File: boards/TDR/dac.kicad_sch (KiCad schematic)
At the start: 9 parts, among them U15 MCP4822, U4 TLV3541

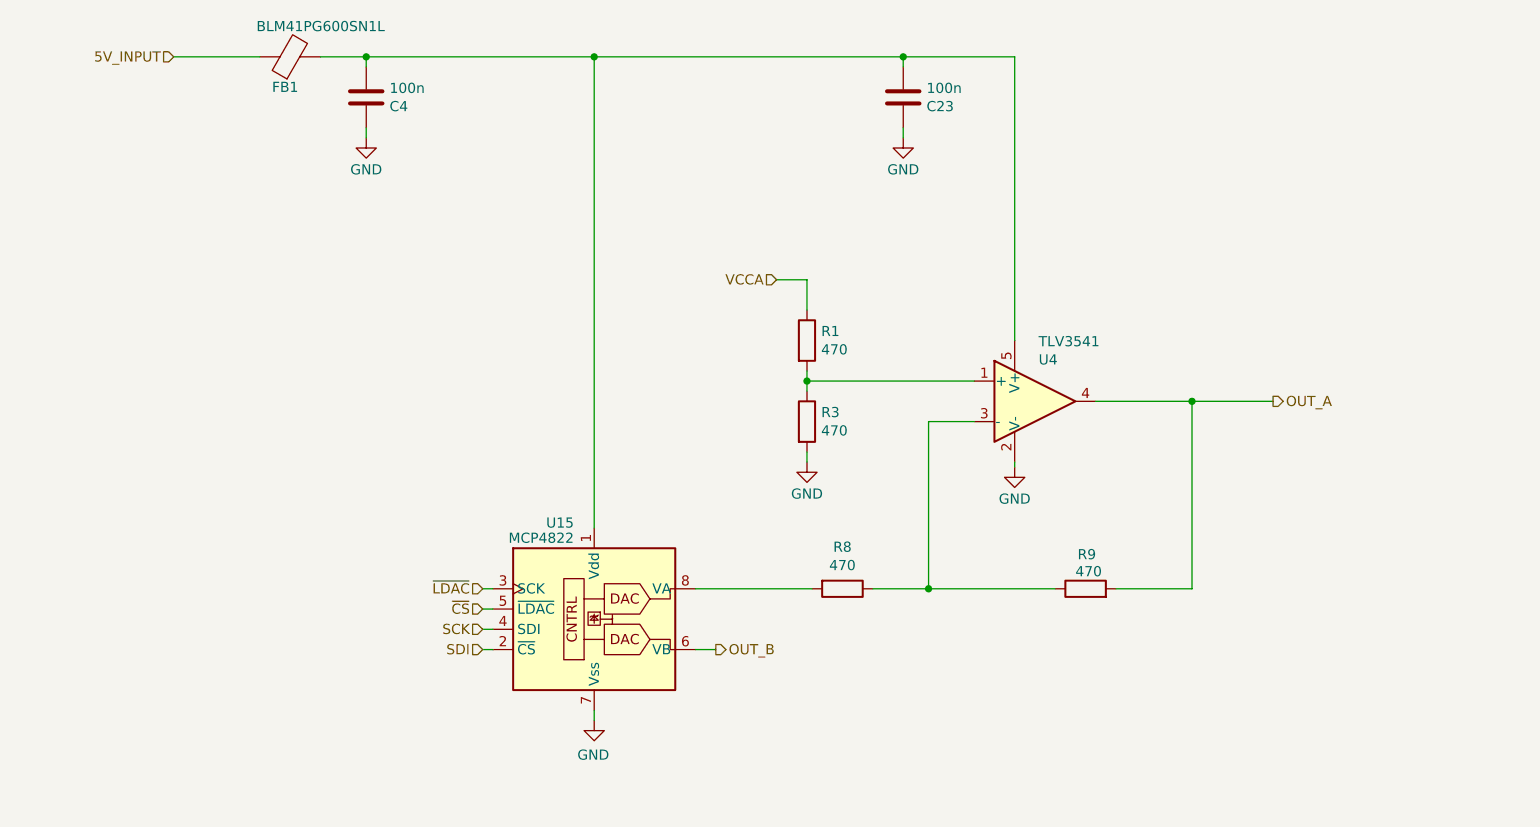
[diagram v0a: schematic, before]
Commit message: hopefully PCB is done
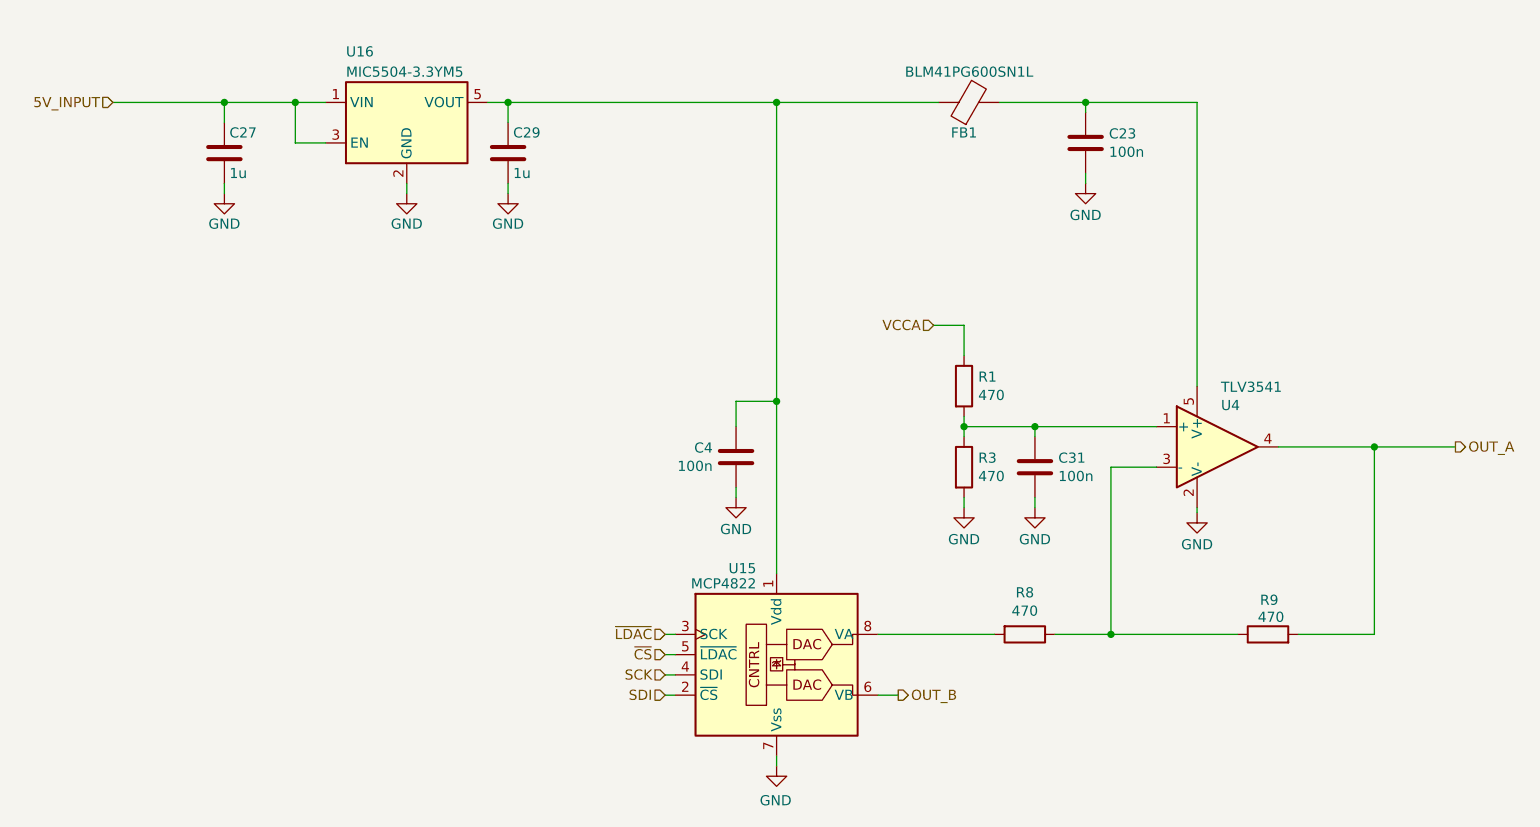
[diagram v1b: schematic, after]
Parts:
- added C27, C29: 1u, Capacitor_SMD:C_0805_2012Metric, symbol Device:C
- added C31: 100n, Capacitor_SMD:C_0402_1005Metric, symbol Device:C
- added U16: MIC5504-3.3YM5, Package_TO_SOT_SMD:SOT-23-5, symbol Regulator_Linear:MIC5504-3.3YM5
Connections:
- net 5V_INPUT: now also C27.1, U16.1 (VIN), U16.3 (EN); no longer FB1.1
- net GND: now also C27.2, C29.2, C31.1, U16.2 (GND)
- net at R1.2, R3.1, U4.1 (+): now also C31.2
- net at C23.1, FB1.2, U4.5 (V+): no longer C4.1, U15.1 (Vdd)
- new net: C29.1, C4.1, FB1.1, U15.1 (Vdd), U16.5 (VOUT)
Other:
- moved on the sheet: C23, C4, FB1, R1, R3, R8, R9, U15, U4
